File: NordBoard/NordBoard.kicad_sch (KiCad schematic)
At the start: 21 parts, among them SW1 SW_Push, SW10 SW_Push, SW11 SW_Push, SW12 SW_Push, SW13 SW_Push, SW14 SW_Push, SW16 SW_Push, SW17 SW_Push, SW18 SW_Push, SW19 SW_Push, SW2 SW_Push, SW20 SW_Push, SW21 SW_Push, SW3 SW_Push, SW4 SW_Push, SW5 SW_Push, SW6 SW_Push, SW7 SW_Push, SW8 SW_Push, SW9 SW_Push, U1 MOUDLE-SEEEDUINO-XIAO

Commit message: feat: PCB
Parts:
- SW1, SW10, SW11, SW12, SW13, SW14, SW16, SW17, SW18, SW19, SW2, SW20, SW21, SW3, SW4, SW5, SW6, SW7, SW8, SW9: footprint PCM_Switch_Keyboard_Hotswap_Kailh:SW_Hotswap_Kailh_Choc_V1V2 -> PCM_marbastlib-choc:SW_choc_v1_1u
- U1: footprint (none) -> Seeed Studio XIAO Series Library:XIAO-RP2040-DIP
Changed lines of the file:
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@@
 			)
 		)
-		(property "Footprint" "PCM_Switch_Keyboard_Hotswap_Kailh:SW_Hotswap_Kailh_Choc_V1V2"
+		(property "Footprint" "PCM_marbastlib-choc:SW_choc_v1_1u"
 			(at 161.29 62.23 0)
 			(effects
@@
 			)
 		)
-		(property "Footprint" "PCM_Switch_Keyboard_Hotswap_Kailh:SW_Hotswap_Kailh_Choc_V1V2"
+		(property "Footprint" "PCM_marbastlib-choc:SW_choc_v1_1u"
 			(at 92.71 59.69 0)
 			(effects
@@
 			)
 		)
-		(property "Footprint" "PCM_Switch_Keyboard_Hotswap_Kailh:SW_Hotswap_Kailh_Choc_V1V2"
+		(property "Footprint" "PCM_marbastlib-choc:SW_choc_v1_1u"
 			(at 46.99 60.96 0)
 			(effects
@@
 			)
 		)
-		(property "Footprint" "PCM_Switch_Keyboard_Hotswap_Kailh:SW_Hotswap_Kailh_Choc_V1V2"
+		(property "Footprint" "PCM_marbastlib-choc:SW_choc_v1_1u"
 			(at 115.57 54.61 0)
 			(effects
@@
 			)
 		)
-		(property "Footprint" ""
+		(property "Footprint" "Seeed Studio XIAO Series Library:XIAO-RP2040-DIP"
 			(at 213.36 46.99 0)
 			(effects
@@
 			)
 		)
-		(property "Footprint" "PCM_Switch_Keyboard_Hotswap_Kailh:SW_Hotswap_Kailh_Choc_V1V2"
+		(property "Footprint" "PCM_marbastlib-choc:SW_choc_v1_1u"
 			(at 161.29 36.83 0)
 			(effects
@@
 			)
 		)
-		(property "Footprint" "PCM_Switch_Keyboard_Hotswap_Kailh:SW_Hotswap_Kailh_Choc_V1V2"
+		(property "Footprint" "PCM_marbastlib-choc:SW_choc_v1_1u"
 			(at 115.57 29.21 0)
 			(effects
@@
 			)
 		)
-		(property "Footprint" "PCM_Switch_Keyboard_Hotswap_Kailh:SW_Hotswap_Kailh_Choc_V1V2"
+		(property "Footprint" "PCM_marbastlib-choc:SW_choc_v1_1u"
 			(at 161.29 49.53 0)
 			(effects
@@
 			)
 		)
-		(property "Footprint" "PCM_Switch_Keyboard_Hotswap_Kailh:SW_Hotswap_Kailh_Choc_V1V2"
+		(property "Footprint" "PCM_marbastlib-choc:SW_choc_v1_1u"
 			(at 69.85 39.37 0)
 			(effects
@@
 			)
 		)
-		(property "Footprint" "PCM_Switch_Keyboard_Hotswap_Kailh:SW_Hotswap_Kailh_Choc_V1V2"
+		(property "Footprint" "PCM_marbastlib-choc:SW_choc_v1_1u"
 			(at 92.71 34.29 0)
 			(effects
@@
 			)
 		)
-		(property "Footprint" "PCM_Switch_Keyboard_Hotswap_Kailh:SW_Hotswap_Kailh_Choc_V1V2"
+		(property "Footprint" "PCM_marbastlib-choc:SW_choc_v1_1u"
 			(at 69.85 64.77 0)
 			(effects
@@
 			)
 		)
-		(property "Footprint" "PCM_Switch_Keyboard_Hotswap_Kailh:SW_Hotswap_Kailh_Choc_V1V2"
+		(property "Footprint" "PCM_marbastlib-choc:SW_choc_v1_1u"
 			(at 184.15 64.77 0)
 			(effects
@@
 			)
 		)
-		(property "Footprint" "PCM_Switch_Keyboard_Hotswap_Kailh:SW_Hotswap_Kailh_Choc_V1V2"
+		(property "Footprint" "PCM_marbastlib-choc:SW_choc_v1_1u"
 			(at 92.71 46.99 0)
 			(effects
@@
 			)
 		)
-		(property "Footprint" "PCM_Switch_Keyboard_Hotswap_Kailh:SW_Hotswap_Kailh_Choc_V1V2"
+		(property "Footprint" "PCM_marbastlib-choc:SW_choc_v1_1u"
 			(at 138.43 33.02 0)
 			(effects
@@
 			)
 		)
-		(property "Footprint" "PCM_Switch_Keyboard_Hotswap_Kailh:SW_Hotswap_Kailh_Choc_V1V2"
+		(property "Footprint" "PCM_marbastlib-choc:SW_choc_v1_1u"
 			(at 138.43 58.42 0)
 			(effects
@@
 			)
 		)
-		(property "Footprint" "PCM_Switch_Keyboard_Hotswap_Kailh:SW_Hotswap_Kailh_Choc_V1V2"
+		(property "Footprint" "PCM_marbastlib-choc:SW_choc_v1_1u"
 			(at 184.15 39.37 0)
 			(effects
@@
 			)
 		)
-		(property "Footprint" "PCM_Switch_Keyboard_Hotswap_Kailh:SW_Hotswap_Kailh_Choc_V1V2"
+		(property "Footprint" "PCM_marbastlib-choc:SW_choc_v1_1u"
 			(at 184.15 52.07 0)
 			(effects
@@
 			)
 		)
-		(property "Footprint" "PCM_Switch_Keyboard_Hotswap_Kailh:SW_Hotswap_Kailh_Choc_V1V2"
+		(property "Footprint" "PCM_marbastlib-choc:SW_choc_v1_1u"
 			(at 46.99 48.26 0)
 			(effects
@@
 			)
 		)
-		(property "Footprint" "PCM_Switch_Keyboard_Hotswap_Kailh:SW_Hotswap_Kailh_Choc_V1V2"
+		(property "Footprint" "PCM_marbastlib-choc:SW_choc_v1_1u"
 			(at 115.57 41.91 0)
 			(effects
@@
 			)
 		)
-		(property "Footprint" "PCM_Switch_Keyboard_Hotswap_Kailh:SW_Hotswap_Kailh_Choc_V1V2"
+		(property "Footprint" "PCM_marbastlib-choc:SW_choc_v1_1u"
 			(at 138.43 45.72 0)
 			(effects
@@
 			)
 		)
-		(property "Footprint" "PCM_Switch_Keyboard_Hotswap_Kailh:SW_Hotswap_Kailh_Choc_V1V2"
+		(property "Footprint" "PCM_marbastlib-choc:SW_choc_v1_1u"
 			(at 69.85 52.07 0)
 			(effects

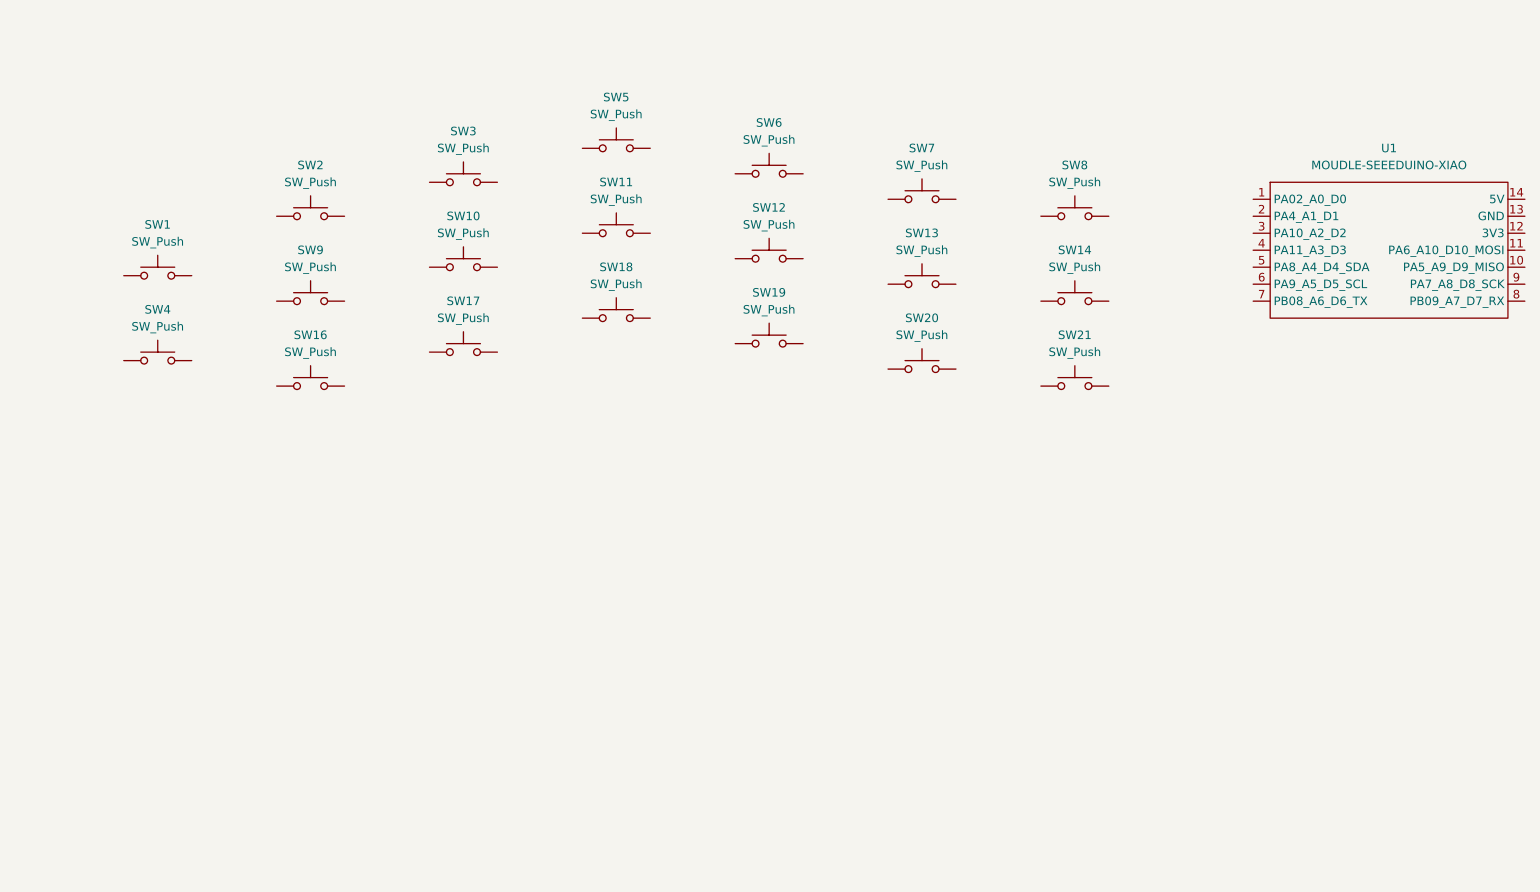
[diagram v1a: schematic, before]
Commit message: feat: work on schem layout
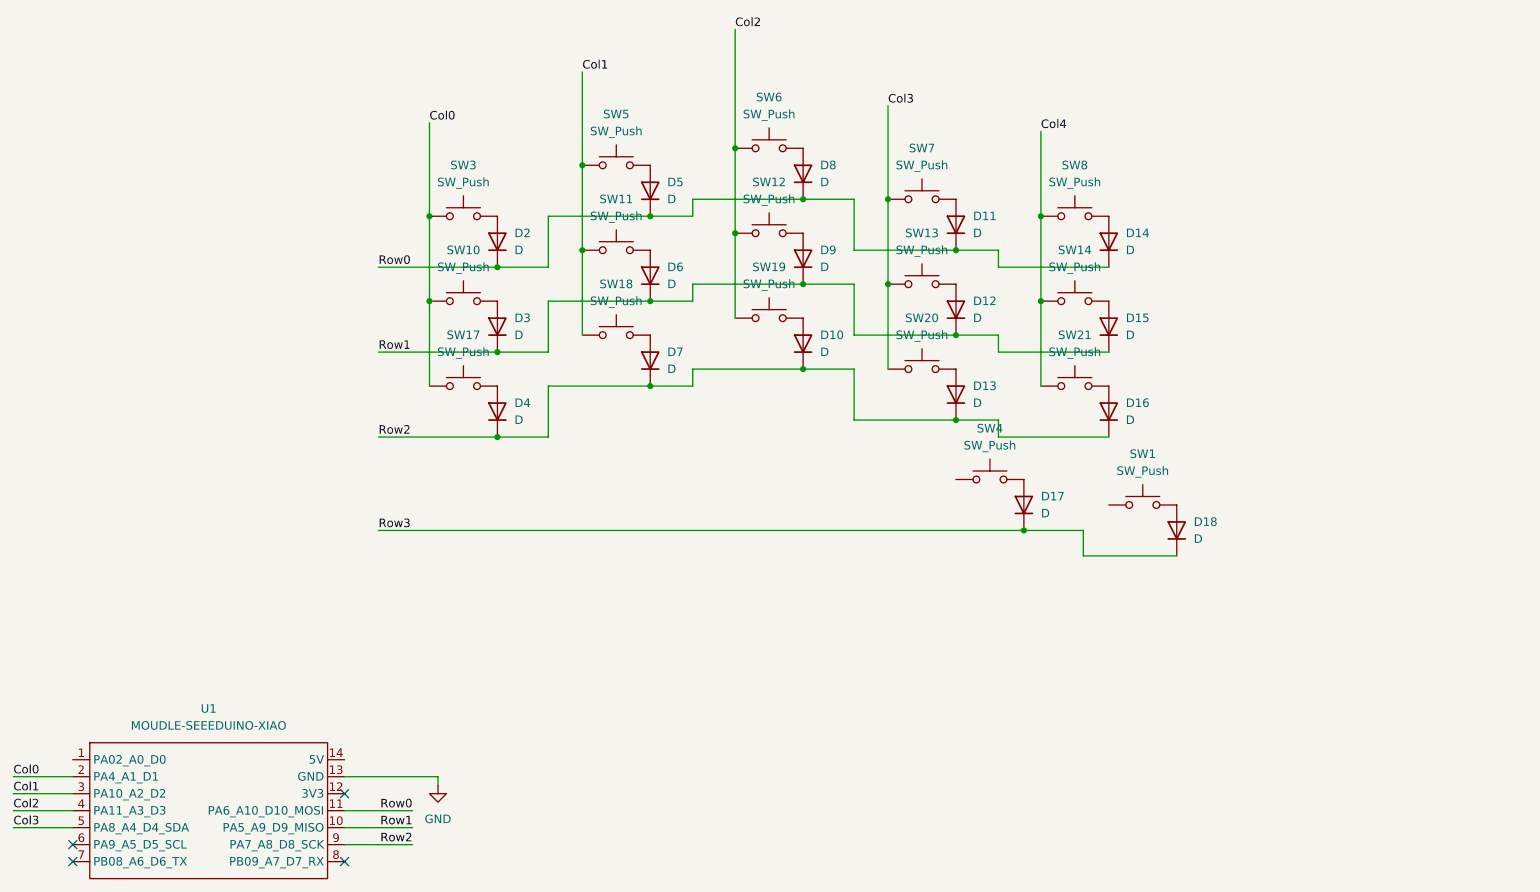
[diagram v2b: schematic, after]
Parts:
- removed SW16, SW2, SW9: SW_Push, PCM_marbastlib-choc:SW_choc_v1_1u, symbol Switch:SW_Push
- added D10, D11, D12, D13, D14, D15, D16, D17, D18, D2, D3, D4, D5, D6, D7, D8, D9: D, symbol Device:D
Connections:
- net Col3: now reaches SW20.1
- net Col3: now also SW13.1, SW7.1, U1.5 (PA8_A4_D4_SDA)
- net at SW20.2: now also D13.2 (A)
- net Col0: now reaches SW17.1
- net Col0: now also SW10.1, SW3.1, U1.2 (PA4_A1_D1)
- net at SW17.2: now also D4.2 (A)
- net at SW4.2: now also D17.2 (A)
- net Col1: now reaches SW18.1
- net Col1: now also SW11.1, SW5.1, U1.3 (PA10_A2_D2)
- net at SW18.2: now also D7.2 (A)
- net Row1: now reaches U1.10 (PA5_A9_D9_MISO)
- net Row1: now also D12.1 (K), D15.1 (K), D3.1 (K), D6.1 (K), D9.1 (K)
- net Row0: now reaches U1.11 (PA6_A10_D10_MOSI)
- net Row0: now also D11.1 (K), D14.1 (K), D2.1 (K), D5.1 (K), D8.1 (K)
- net GND: now reaches U1.13 (GND)
- net Col2: now reaches U1.4 (PA11_A3_D3)
- net Col2: now also SW12.1, SW19.1, SW6.1
- net Row2: now reaches U1.9 (PA7_A8_D8_SCK)
- net Row2: now also D10.1 (K), D13.1 (K), D16.1 (K), D4.1 (K), D7.1 (K)
- net at SW7.2: now also D11.2 (A)
- net at SW5.2: now also D5.2 (A)
- net at SW13.2: now also D12.2 (A)
- net at SW3.2: now also D2.2 (A)
- net Col4: now reaches SW21.1
- net Col4: now also SW14.1, SW8.1
- net at SW21.2: now also D16.2 (A)
- net at SW10.2: now also D3.2 (A)
- net at SW6.2: now also D8.2 (A)
- net at SW19.2: now also D10.2 (A)
- net at SW8.2: now also D14.2 (A)
- net at SW14.2: now also D15.2 (A)
- net at SW1.2: now also D18.2 (A)
- net at SW11.2: now also D6.2 (A)
- net at SW12.2: now also D9.2 (A)
- new net Row3: D17.1 (K), D18.1 (K)
- no-connect marks 0 -> 4
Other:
- moved on the sheet: SW1, SW10, SW11, SW12, SW17, SW18, SW19, SW3, SW4, SW5, SW6, U1

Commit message: feat: schem
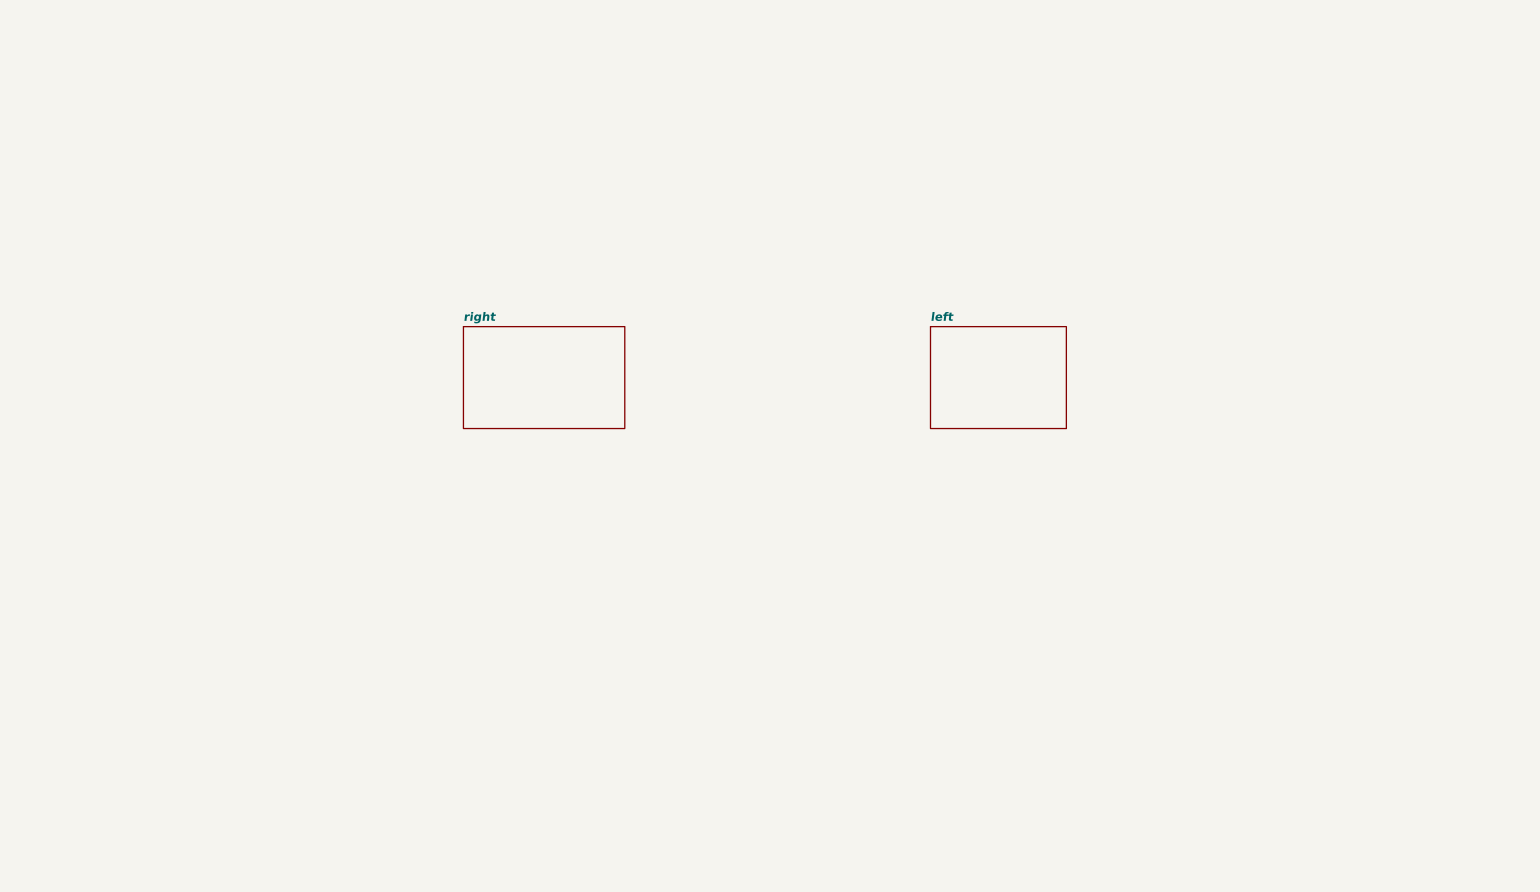
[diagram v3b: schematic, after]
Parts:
- removed D10, D11, D12, D13, D14, D15, D16, D17, D18, D2, D3, D4, D5, D6, D7, D8, D9: D, symbol Device:D
- removed SW1, SW10, SW11, SW12, SW13, SW14, SW17, SW18, SW19, SW20, SW21, SW3, SW4, SW5, SW6, SW7, SW8: SW_Push, PCM_marbastlib-choc:SW_choc_v1_1u, symbol Switch:SW_Push
- removed U1: MOUDLE-SEEEDUINO-XIAO, Seeed Studio XIAO Series Library:XIAO-RP2040-DIP, symbol XIAO_RP2040:MOUDLE-SEEEDUINO-XIAO
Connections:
- no-connect marks 4 -> 0
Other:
- added sheet left (side.kicad_sch)
- added sheet right (right.kicad_sch)
